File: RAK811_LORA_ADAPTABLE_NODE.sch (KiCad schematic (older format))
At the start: 18 parts, among them J1 Screw_Terminal_01x02, J2 Screw_Terminal_01x03, J3 Conn_01x01_Male, J4 Conn_01x01_Male, J5 Conn_01x01_Male, J6 Conn_01x01_Male, J7 Conn_Coaxial, U1 RAK811-HF

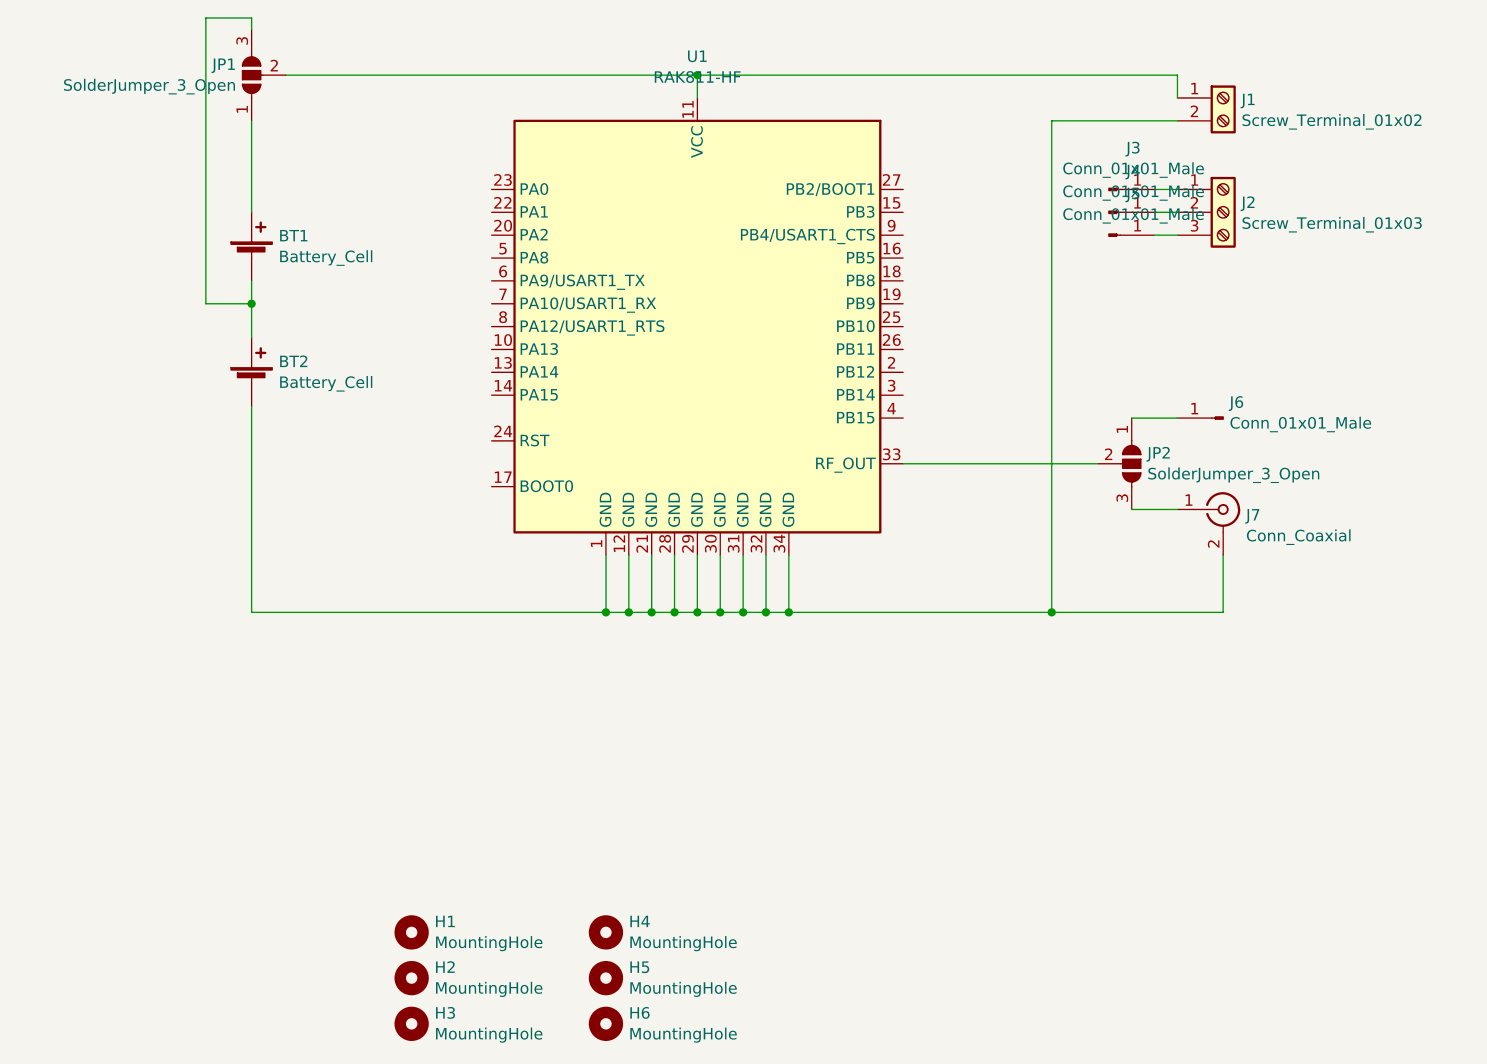
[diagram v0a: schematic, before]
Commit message: some i/o pins layout
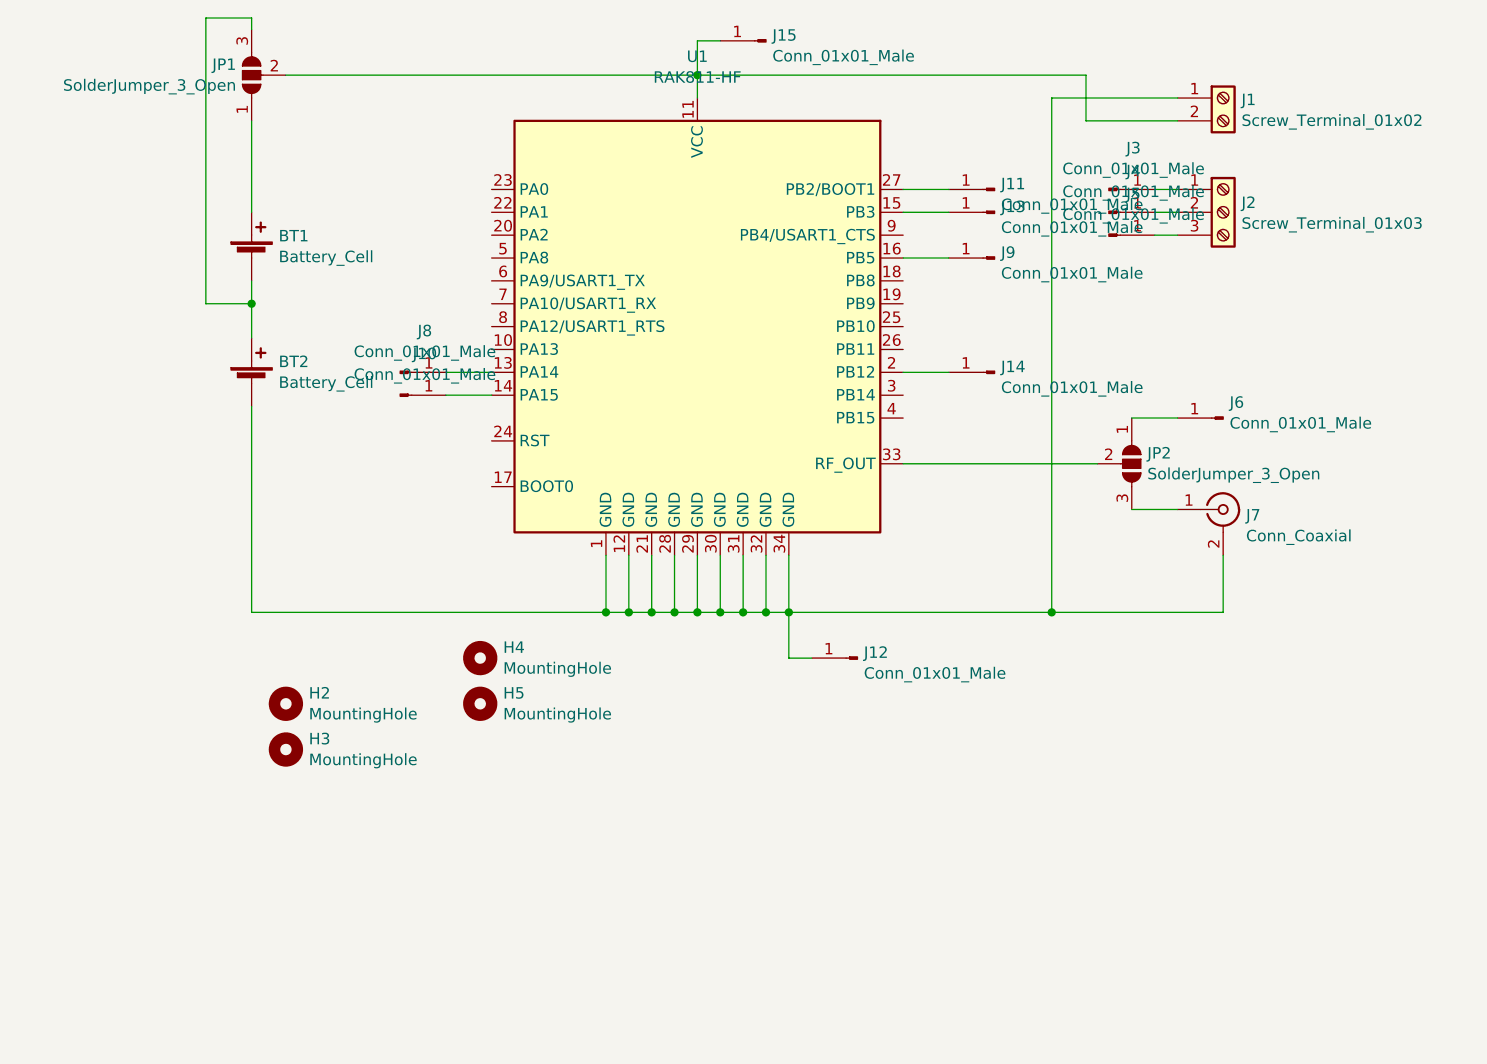
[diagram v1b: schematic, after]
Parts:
- removed H1, H6: MountingHole, MountingHole:MountingHole_3mm, symbol Mechanical:MountingHole
- added J10, J11, J12, J13, J14, J15, J8, J9: Conn_01x01_Male, Connector_Wire:SolderWirePad_1x01_Drill0.8mm, symbol Connector:Conn_01x01_Male
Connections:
- net at BT2.2 (-), J7.2 (Ext), U1.1 (GND)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: now also J1.1 (Pin_1), J12.1 (Pin_1); no longer J1.2 (Pin_2)
- net at JP1.2 (C), U1.11 (VCC): now also J1.2 (Pin_2), J15.1 (Pin_1); no longer J1.1 (Pin_1)
- net at U1.13 (PA14): now also J8.1 (Pin_1)
- net at U1.14 (PA15): now also J10.1 (Pin_1)
- net at U1.15 (PB3): now also J13.1 (Pin_1)
- net at U1.16 (PB5): now also J9.1 (Pin_1)
- net at U1.2 (PB12): now also J14.1 (Pin_1)
- net at U1.27 (PB2/BOOT1): now also J11.1 (Pin_1)
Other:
- moved on the sheet: H2, H3, H4, H5
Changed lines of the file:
@@
 $EndDescr
-$Comp
-L Mechanical:MountingHole H1
-U 1 1 5EED2AEB
-P 4200 5600
-F 0 "H1" H 4300 5646 50  0000 L CNN
-F 1 "MountingHole" H 4300 5555 50  0000 L CNN
-F 2 "MountingHole:MountingHole_3mm" H 4200 5600 50  0001 C CNN
-F 3 "~" H 4200 5600 50  0001 C CNN
-	1    4200 5600
-	1    0    0    -1
-$EndComp
 $Comp
 L Mechanical:MountingHole H2
 U 1 1 5EED2E39
-P 4200 5800
-F 0 "H2" H 4300 5846 50  0000 L CNN
-F 1 "MountingHole" H 4300 5755 50  0000 L CNN
-F 2 "MountingHole:MountingHole_3mm" H 4200 5800 50  0001 C CNN
-F 3 "~" H 4200 5800 50  0001 C CNN
-	1    4200 5800
+P 3650 4600
+F 0 "H2" H 3750 4646 50  0000 L CNN
+F 1 "MountingHole" H 3750 4555 50  0000 L CNN
+F 2 "MountingHole:MountingHole_3mm" H 3650 4600 50  0001 C CNN
+F 3 "~" H 3650 4600 50  0001 C CNN
+	1    3650 4600
 	1    0    0    -1
 $EndComp
@@
 L Mechanical:MountingHole H3
 U 1 1 5EED3144
-P 4200 6000
-F 0 "H3" H 4300 6046 50  0000 L CNN
-F 1 "MountingHole" H 4300 5955 50  0000 L CNN
-F 2 "MountingHole:MountingHole_3mm" H 4200 6000 50  0001 C CNN
-F 3 "~" H 4200 6000 50  0001 C CNN
-	1    4200 6000
+P 3650 4800
+F 0 "H3" H 3750 4846 50  0000 L CNN
+F 1 "MountingHole" H 3750 4755 50  0000 L CNN
+F 2 "MountingHole:MountingHole_3mm" H 3650 4800 50  0001 C CNN
+F 3 "~" H 3650 4800 50  0001 C CNN
+	1    3650 4800
 	1    0    0    -1
 $EndComp
@@
 L Mechanical:MountingHole H4
 U 1 1 5EED33AC
-P 5050 5600
-F 0 "H4" H 5150 5646 50  0000 L CNN
-F 1 "MountingHole" H 5150 5555 50  0000 L CNN
-F 2 "MountingHole:MountingHole_3mm" H 5050 5600 50  0001 C CNN
-F 3 "~" H 5050 5600 50  0001 C CNN
-	1    5050 5600
-	1    0    0    -1
-$EndComp
-$Comp
-L Mechanical:MountingHole H6
-U 1 1 5EED36FB
-P 5050 6000
-F 0 "H6" H 5150 6046 50  0000 L CNN
-F 1 "MountingHole" H 5150 5955 50  0000 L CNN
-F 2 "MountingHole:MountingHole_3mm" H 5050 6000 50  0001 C CNN
-F 3 "~" H 5050 6000 50  0001 C CNN
-	1    5050 6000
+P 4500 4400
+F 0 "H4" H 4600 4446 50  0000 L CNN
+F 1 "MountingHole" H 4600 4355 50  0000 L CNN
+F 2 "MountingHole:MountingHole_3mm" H 4500 4400 50  0001 C CNN
+F 3 "~" H 4500 4400 50  0001 C CNN
+	1    4500 4400
 	1    0    0    -1
 $EndComp
@@
 L Mechanical:MountingHole H5
 U 1 1 5EED3A44
-P 5050 5800
-F 0 "H5" H 5150 5846 50  0000 L CNN
-F 1 "MountingHole" H 5150 5755 50  0000 L CNN
-F 2 "MountingHole:MountingHole_3mm" H 5050 5800 50  0001 C CNN
-F 3 "~" H 5050 5800 50  0001 C CNN
-	1    5050 5800
+P 4500 4600
+F 0 "H5" H 4600 4646 50  0000 L CNN
+F 1 "MountingHole" H 4600 4555 50  0000 L CNN
+F 2 "MountingHole:MountingHole_3mm" H 4500 4600 50  0001 C CNN
+F 3 "~" H 4500 4600 50  0001 C CNN
+	1    4500 4600
 	1    0    0    -1
 $EndComp
@@
 $EndComp
 Wire Wire Line
-	7550 1950 7550 1850
-Wire Wire Line
-	7550 1850 5450 1850
-Connection ~ 5450 1850
-Wire Wire Line
-	7550 2050 7000 2050
-Wire Wire Line
-	7000 2050 7000 4200
-Wire Wire Line
 	7000 4200 5850 4200
 Connection ~ 5850 4200
@@
 	7750 4200 7000 4200
 Connection ~ 7000 4200
+Wire Wire Line
+	7550 1950 7000 1950
+Wire Wire Line
+	7000 1950 7000 4200
+Wire Wire Line
+	7550 2050 7150 2050
+Wire Wire Line
+	7150 2050 7150 1850
+Wire Wire Line
+	7150 1850 5450 1850
+Connection ~ 5450 1850
+$Comp
+L Connector:Conn_01x01_Male J8
+U 1 1 5EF586B6
+P 4150 3150
+F 0 "J8" H 4258 3331 50  0000 C CNN
+F 1 "Conn_01x01_Male" H 4258 3240 50  0000 C CNN
+F 2 "Connector_Wire:SolderWirePad_1x01_Drill0.8mm" H 4150 3150 50  0001 C CNN
+F 3 "~" H 4150 3150 50  0001 C CNN
+	1    4150 3150
+	1    0    0    -1
+$EndComp
+Wire Wire Line
+	4350 3150 4550 3150
+$Comp
+L Connector:Conn_01x01_Male J9
+U 1 1 5EF61769
+P 6750 2650
+F 0 "J9" H 6722 2674 50  0000 R CNN
+F 1 "Conn_01x01_Male" H 6722 2583 50  0000 R CNN
+F 2 "Connector_Wire:SolderWirePad_1x01_Drill0.8mm" H 6750 2650 50  0001 C CNN
+F 3 "~" H 6750 2650 50  0001 C CNN
+	1    6750 2650
+	-1   0    0    -1
+$EndComp
+$Comp
+L Connector:Conn_01x01_Male J10
+U 1 1 5EF6CBB4
+P 4150 3250
+F 0 "J10" H 4258 3431 50  0000 C CNN
+F 1 "Conn_01x01_Male" H 4258 3340 50  0000 C CNN
+F 2 "Connector_Wire:SolderWirePad_1x01_Drill0.8mm" H 4150 3250 50  0001 C CNN
+F 3 "~" H 4150 3250 50  0001 C CNN
+	1    4150 3250
+	1    0    0    -1
+$EndComp
+Wire Wire Line
+	4350 3250 4550 3250
+$Comp
+L Connector:Conn_01x01_Male J11
+U 1 1 5EF78D3D
+P 6750 2350
+F 0 "J11" H 6722 2374 50  0000 R CNN
+F 1 "Conn_01x01_Male" H 6722 2283 50  0000 R CNN
+F 2 "Connector_Wire:SolderWirePad_1x01_Drill0.8mm" H 6750 2350 50  0001 C CNN
+F 3 "~" H 6750 2350 50  0001 C CNN
+	1    6750 2350
+	-1   0    0    -1
+$EndComp
+$Comp
+L Connector:Conn_01x01_Male J12
+U 1 1 5EF83DA7
+P 6150 4400
+F 0 "J12" H 6122 4424 50  0000 R CNN
+F 1 "Conn_01x01_Male" H 6122 4333 50  0000 R CNN
+F 2 "Connector_Wire:SolderWirePad_1x01_Drill0.8mm" H 6150 4400 50  0001 C CNN
+F 3 "~" H 6150 4400 50  0001 C CNN
+	1    6150 4400
+	-1   0    0    -1
+$EndComp
+Wire Wire Line
+	5950 4400 5850 4400
+Wire Wire Line
+	5850 4400 5850 4200
+$Comp
+L Connector:Conn_01x01_Male J13
+U 1 1 5EF91077
+P 6750 2450
+F 0 "J13" H 6722 2474 50  0000 R CNN
+F 1 "Conn_01x01_Male" H 6722 2383 50  0000 R CNN
+F 2 "Connector_Wire:SolderWirePad_1x01_Drill0.8mm" H 6750 2450 50  0001 C CNN
+F 3 "~" H 6750 2450 50  0001 C CNN
+	1    6750 2450
+	-1   0    0    -1
+$EndComp
+Wire Wire Line
+	6350 2450 6550 2450
+$Comp
+L Connector:Conn_01x01_Male J14
+U 1 1 5EF9D3AA
+P 6750 3150
+F 0 "J14" H 6722 3174 50  0000 R CNN
+F 1 "Conn_01x01_Male" H 6722 3083 50  0000 R CNN
+F 2 "Connector_Wire:SolderWirePad_1x01_Drill0.8mm" H 6750 3150 50  0001 C CNN
+F 3 "~" H 6750 3150 50  0001 C CNN
+	1    6750 3150
+	-1   0    0    -1
+$EndComp
+Wire Wire Line
+	6350 3150 6550 3150
+$Comp
+L Connector:Conn_01x01_Male J15
+U 1 1 5EFB7B96
+P 5750 1700
+F 0 "J15" H 5722 1724 50  0000 R CNN
+F 1 "Conn_01x01_Male" H 5722 1633 50  0000 R CNN
+F 2 "Connector_Wire:SolderWirePad_1x01_Drill0.8mm" H 5750 1700 50  0001 C CNN
+F 3 "~" H 5750 1700 50  0001 C CNN
+	1    5750 1700
+	-1   0    0    -1
+$EndComp
+Wire Wire Line
+	5550 1700 5450 1700
+Wire Wire Line
+	5450 1700 5450 1850
+Wire Wire Line
+	6350 2350 6550 2350
+Wire Wire Line
+	6350 2650 6550 2650
 $EndSCHEMATC
